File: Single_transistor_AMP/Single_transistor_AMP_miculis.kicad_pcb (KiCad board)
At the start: 2 copper layers, 38.1 x 25.4 mm, 10 parts, among them J1 Conn_01x02, J2 Conn_01x02, Q1 BC548

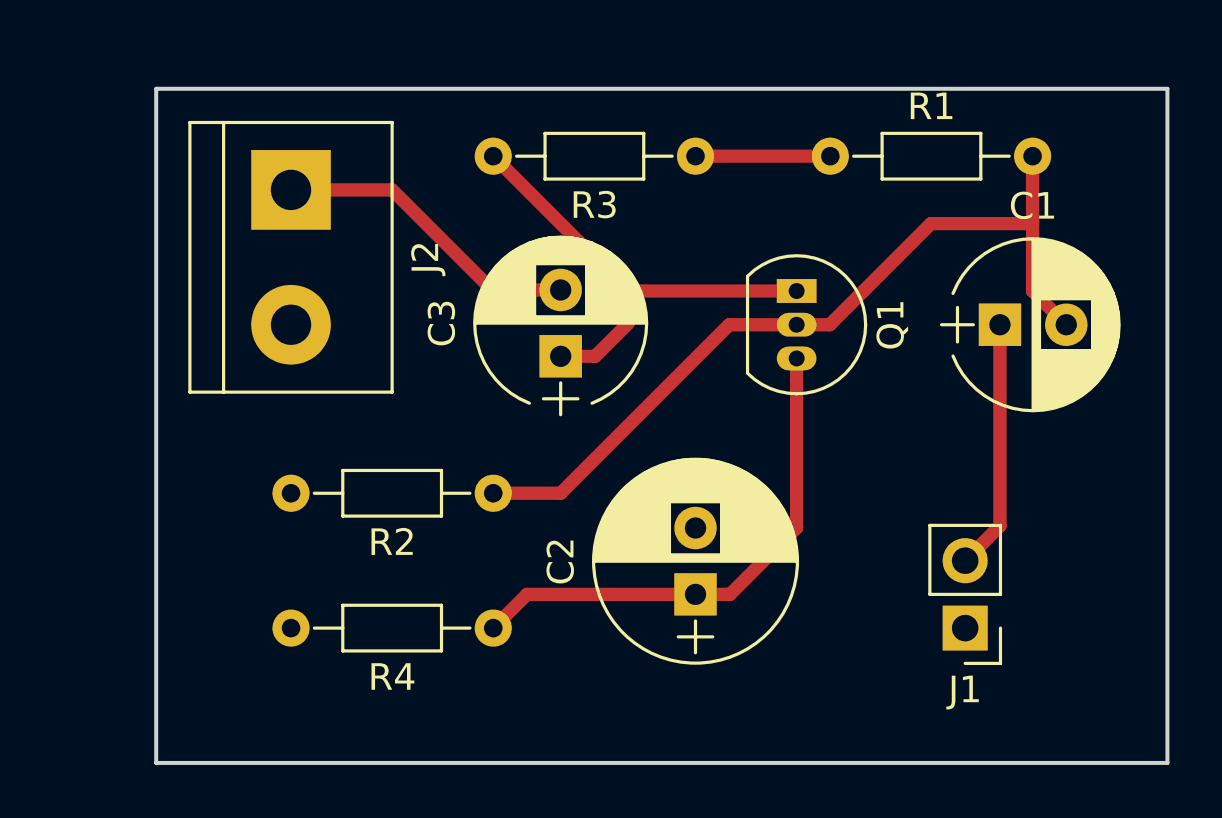
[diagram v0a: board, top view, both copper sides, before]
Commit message: Majas darbi
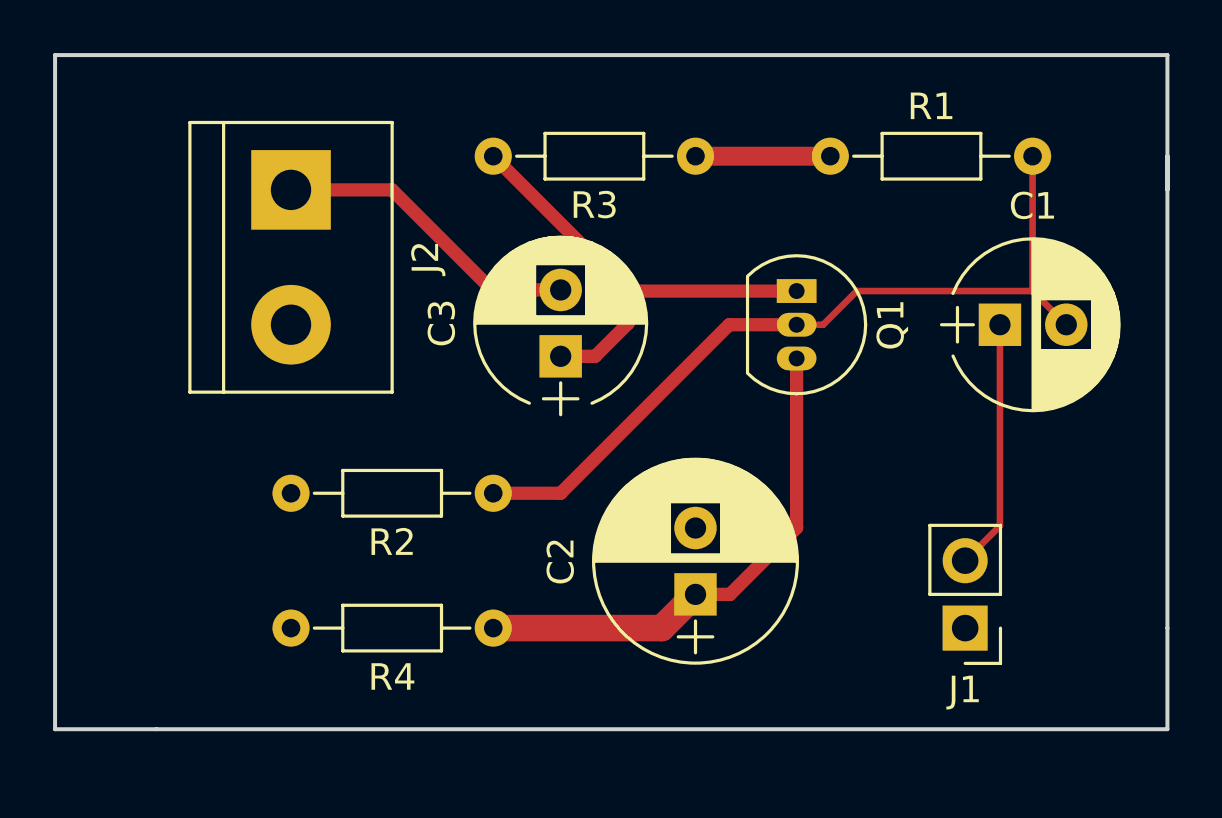
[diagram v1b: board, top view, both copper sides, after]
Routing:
- net Net-(C1-Pad2): track 31.4 -> 30.4 mm
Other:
- board size 38.1 x 25.4 mm -> 41.9 x 25.4 mm
- net class Power added: clearance 0.2, trace_width 0.71, via_dia 0.6, via_drill 0.4
